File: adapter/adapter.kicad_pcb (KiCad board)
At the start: 2 copper layers, 43.5 x 38.6 mm, 15 parts, among them J1 Conn_01x03_Female, J2 Conn_01x06_Female, SW1 RotaryEncoder_Switch

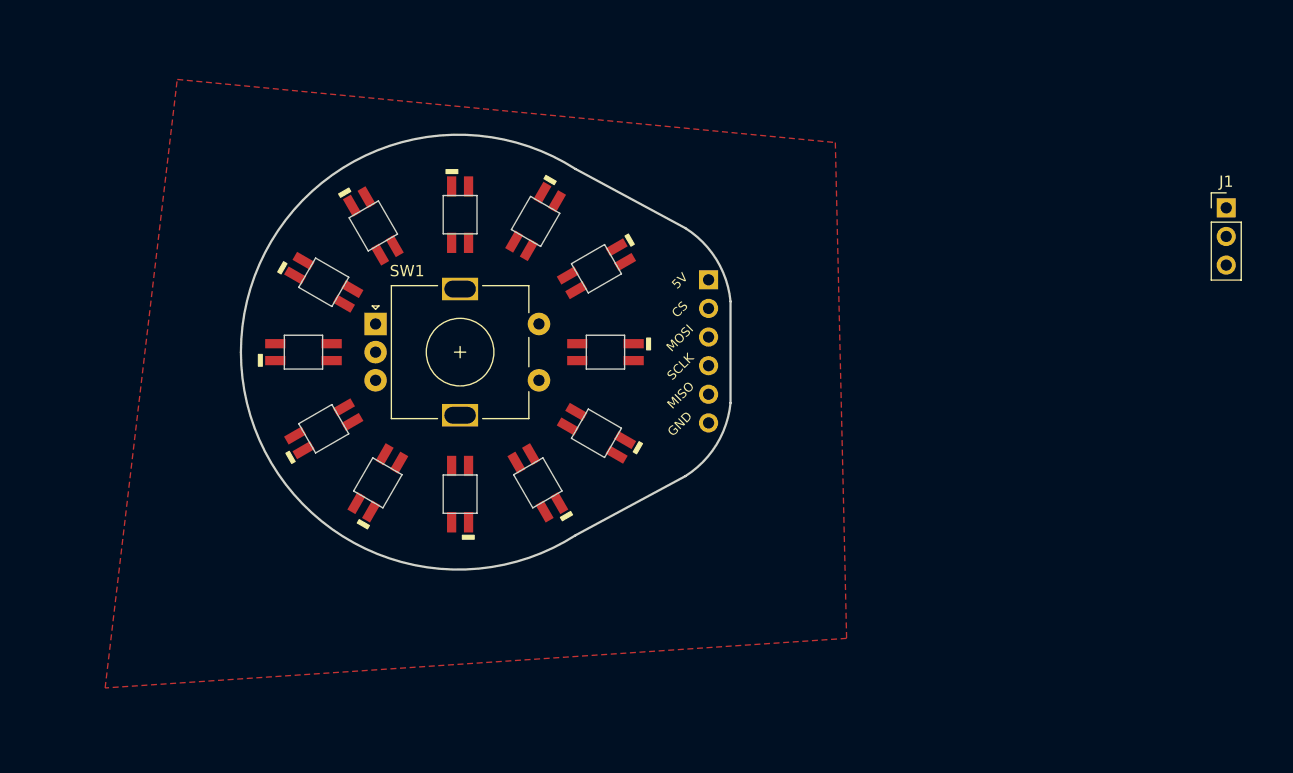
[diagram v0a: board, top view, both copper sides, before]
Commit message: routing
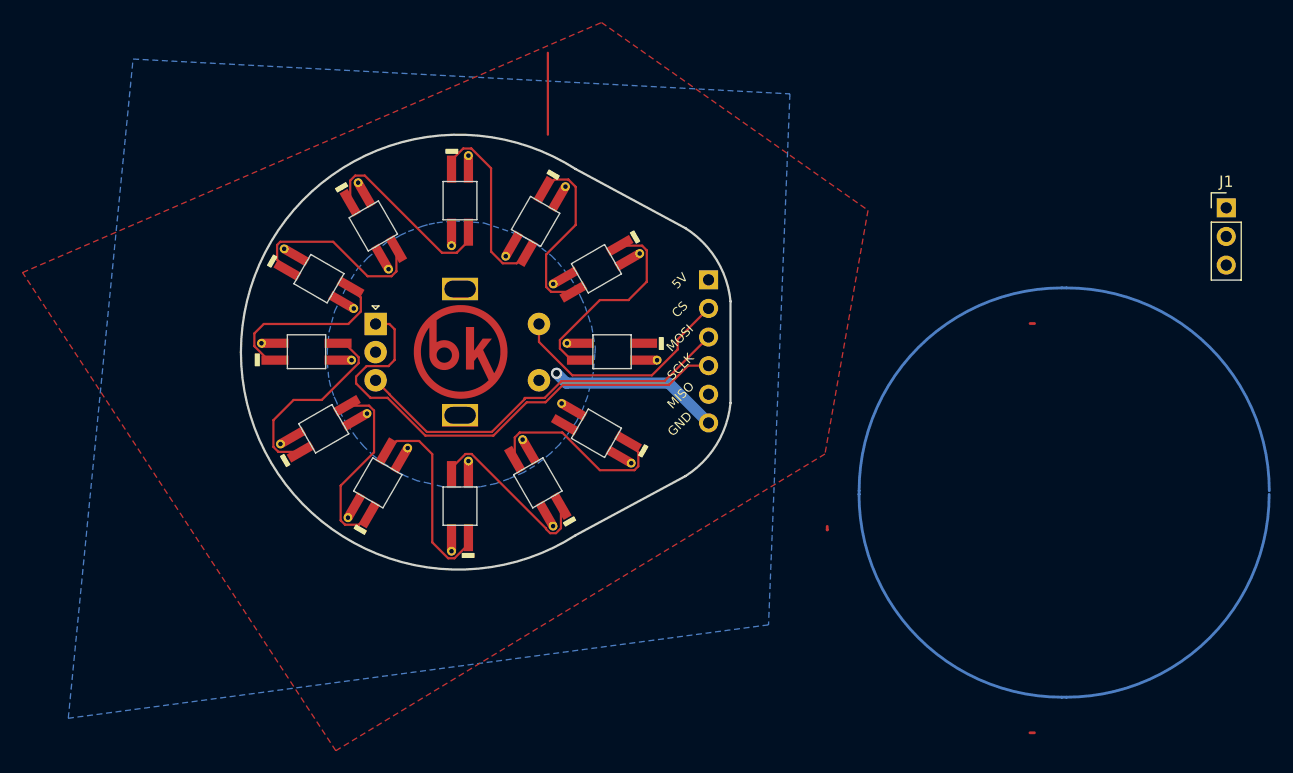
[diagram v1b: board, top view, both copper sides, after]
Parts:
- added G*** (x2): LOGO, LOGO, F.Cu at (52.5, 43.6)
- moved D2 1.24 mm to (52.5, 30.2)
- moved D8 1.07 mm to (52.5, 57.3)
- moved D1 0.58 mm to (66.0, 43.6)
- moved D6 0.53 mm to (40.0, 37.1)
- moved D10 0.27 mm to (38.9, 43.6)
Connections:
- net er renamed button
- D10 pad 1: unconnected-(D10-Pad1) -> Net-(D12-Pad3)
- D10 pad 2: unconnected-(D10-Pad2) -> Gnd
- D10 pad 3: unconnected-(D10-Pad3) -> Net-(D10-Pad3)
- D10 pad 4: unconnected-(D10-Pad4) -> Vcc
- D11 pad 2: unconnected-(D11-Pad2) -> Gnd
- D11 pad 3: unconnected-(D11-Pad3) -> Net-(D11-Pad3)
- D11 pad 4: unconnected-(D11-Pad4) -> Vcc
- D12 pad 1: unconnected-(D12-Pad1) -> Net-(D12-Pad1)
- D12 pad 2: unconnected-(D12-Pad2) -> Gnd
- D12 pad 3: unconnected-(D12-Pad3) -> Net-(D12-Pad3)
- D12 pad 4: unconnected-(D12-Pad4) -> Vcc
- D2 pad 1: unconnected-(D2-Pad1) -> Net-(D4-Pad3)
- D2 pad 2: unconnected-(D2-Pad2) -> Gnd
- D2 pad 3: unconnected-(D2-Pad3) -> Net-(D2-Pad3)
- D2 pad 4: unconnected-(D2-Pad4) -> Vcc
- D4 pad 1: unconnected-(D4-Pad1) -> Net-(D4-Pad1)
- D4 pad 2: unconnected-(D4-Pad2) -> Gnd
- D4 pad 3: unconnected-(D4-Pad3) -> Net-(D4-Pad3)
- D4 pad 4: unconnected-(D4-Pad4) -> Vcc
- D5 pad 1: unconnected-(D5-Pad1) -> Net-(D2-Pad3)
- D6 pad 1: unconnected-(D6-Pad1) -> Net-(D10-Pad3)
- D6 pad 2: unconnected-(D6-Pad2) -> Gnd
- D6 pad 3: unconnected-(D6-Pad3) -> Net-(D4-Pad1)
- D6 pad 4: unconnected-(D6-Pad4) -> Vcc
- D7 pad 1: unconnected-(D7-Pad1) -> Net-(D7-Pad1)
- D7 pad 2: unconnected-(D7-Pad2) -> Gnd
- D7 pad 3: unconnected-(D7-Pad3) -> Net-(D12-Pad1)
- D7 pad 4: unconnected-(D7-Pad4) -> Vcc
- D8 pad 1: unconnected-(D8-Pad1) -> Net-(D8-Pad1)
- D8 pad 2: unconnected-(D8-Pad2) -> Gnd
- D8 pad 3: unconnected-(D8-Pad3) -> Net-(D7-Pad1)
- D8 pad 4: unconnected-(D8-Pad4) -> Vcc
- D9 pad 1: unconnected-(D9-Pad1) -> Net-(D11-Pad3)
- D9 pad 2: unconnected-(D9-Pad2) -> Gnd
- D9 pad 3: unconnected-(D9-Pad3) -> Net-(D8-Pad1)
- D9 pad 4: unconnected-(D9-Pad4) -> Vcc
- J2 pad 1: +5V -> Vcc
- J2 pad 3: ec -> r1
- J2 pad 4: edb -> r2
- J2 pad 6: GND -> Gnd
- SW1 pad A: eda -> r2
- SW1 pad B: edb -> r1
- SW1 pad C: GND -> Gnd
- SW1 pad S1: ec -> Gnd
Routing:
- net Vcc: track 0.00 -> 111.3 mm
- net r2: track 0.00 -> 45.0 mm
- net r1: track 0.00 -> 35.0 mm
- net button: track 0.00 -> 20.9 mm
- net Net-(D1-Pad1): track 0.00 -> 18.2 mm
- net Net-(D7-Pad1): track 0.00 -> 17.7 mm
- net Net-(D12-Pad3): track 0.00 -> 17.5 mm
- net Net-(D11-Pad3): track 0.00 -> 17.2 mm
- net Net-(D2-Pad3): track 0.00 -> 16.9 mm
- net Net-(D4-Pad1): track 0.00 -> 16.8 mm
- net Net-(D4-Pad3): track 0.00 -> 16.7 mm
- net Net-(D12-Pad1): track 0.00 -> 16.7 mm
- net Net-(D10-Pad3): track 0.00 -> 16.3 mm
- net Net-(D3-Pad1): track 0.00 -> 16.0 mm
- net Net-(D8-Pad1): track 0.00 -> 15.9 mm
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- added copper zone on B.Cu, net Gnd
- added copper zone on F.Cu, net Gnd
- added copper zone on B.Cu, net Vcc
- removed copper zone on F.Cu, net GND
